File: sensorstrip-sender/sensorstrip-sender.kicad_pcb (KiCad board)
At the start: 2 copper layers, 56 x 12 mm, 13 parts, among them J1 USB_C_Receptacle_PowerOnly, J2 Conn_01x02_MountingPin, SW1 SW_DPDT_x2

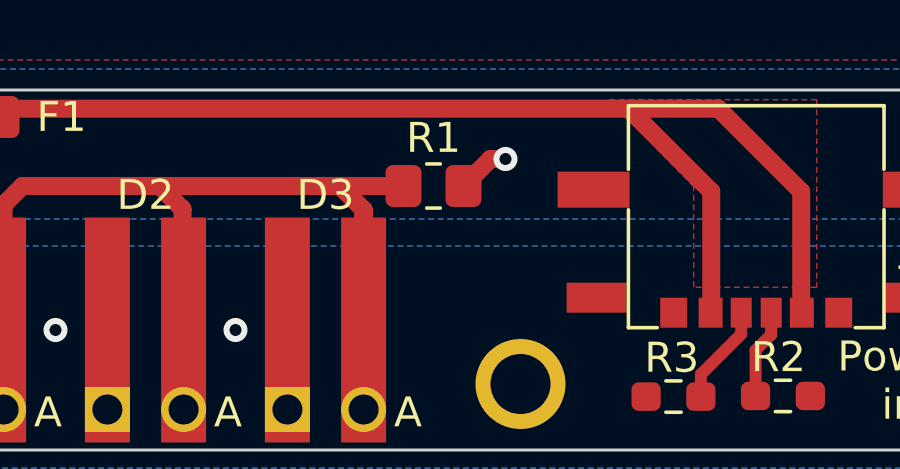
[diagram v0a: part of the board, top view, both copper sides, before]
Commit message: of course i ran drc before pushing what do you take me for
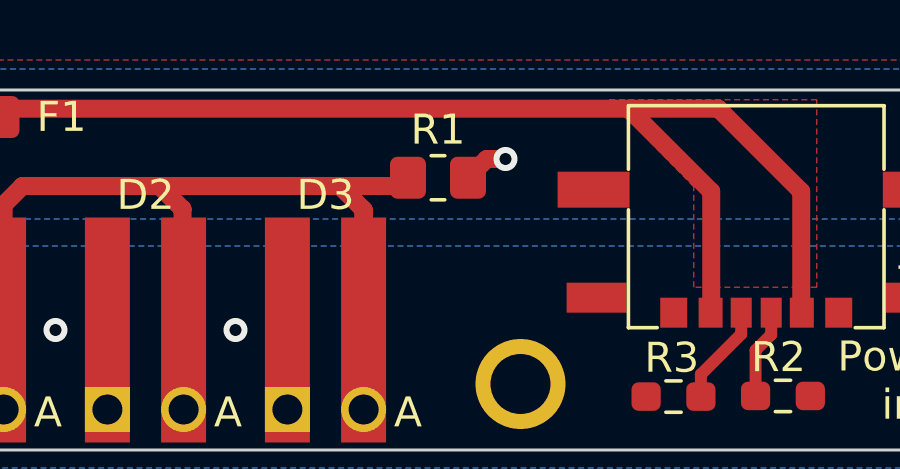
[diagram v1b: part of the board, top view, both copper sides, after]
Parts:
- moved R1 0.31 mm to (137.8, 52.9)
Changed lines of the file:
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@@
   (net 8 "/Power_postFuse")
   (footprint "Resistor_SMD:R_0805_2012Metric_Pad1.20x1.40mm_HandSolder" (layer "F.Cu")
-    (at 137.6 53.2)
+    (at 137.75 52.925)
     (descr "Resistor SMD 0805 (2012 Metric), square (rectangular) end terminal, IPC_7351 nominal with elongated pad for handsoldering. (Body size source: IPC-SM-782 page 72, https://www.pcb-3d.com/wordpress/wp-content/uploads/ipc-sm-782a_amendment_1_and_2.pdf), generated with kicad-footprint-generator")
     (tags "resistor handsolder")
@@
   (segment (start 128.465 53.2) (end 129.235 53.97) (width 0.6) (layer "F.Cu") (net 4))
   (segment (start 135.27 53.99) (end 134.48 53.2) (width 0.6) (layer "F.Cu") (net 4))
+  (segment (start 139.375 52.3) (end 138.75 52.925) (width 0.6) (layer "F.Cu") (net 5))
   (segment (start 115.225 55.6) (end 115.225 53.225) (width 0.6) (layer "F.Cu") (net 5))
   (segment (start 102.53 59.35) (end 102.53 53.85) (width 0.6) (layer "F.Cu") (net 5))
-  (segment (start 140 52.3) (end 139.5 52.3) (width 0.6) (layer "F.Cu") (net 5))
-  (segment (start 139.5 52.3) (end 138.6 53.2) (width 0.6) (layer "F.Cu") (net 5))
   (segment (start 115.225 53.225) (end 114.8 52.8) (width 0.6) (layer "F.Cu") (net 5))
+  (segment (start 140 52.3) (end 139.375 52.3) (width 0.6) (layer "F.Cu") (net 5))
   (segment (start 102.7 53.25) (end 102.7 51.4) (width 0.6) (layer "F.Cu") (net 5))
   (via (at 102.7 51.4) (size 0.8) (drill 0.4) (layers "F.Cu" "B.Cu") (net 5))
